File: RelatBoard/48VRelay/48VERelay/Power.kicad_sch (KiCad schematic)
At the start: 25 parts, among them J1 12, U4 3A 32V, U5 TPS630701RNMR, U7 AP7343DQ-33W5-7, U8 AP7343DQ-33W5-7

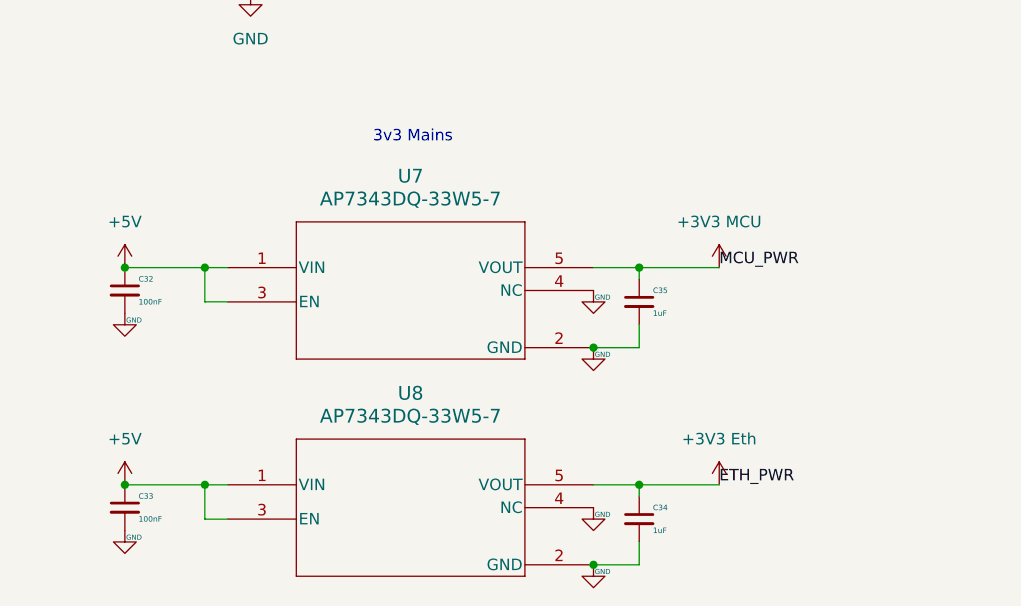
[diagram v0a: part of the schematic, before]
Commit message: begin pcb design
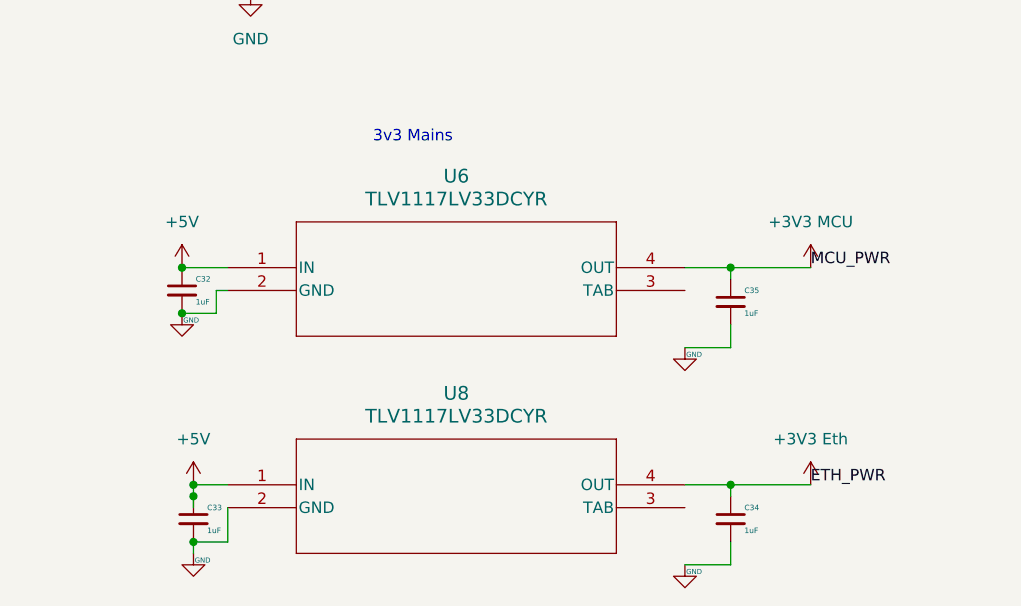
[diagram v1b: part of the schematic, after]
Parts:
- removed U7, U8: AP7343DQ-33W5-7, AP7343DQ-33W5-7_DIO, symbol AP7343DQ-33W5-7:AP7343DQ-33W5-7
- added U6, U8: TLV1117LV33DCYR, YDC4, symbol 2026-06-15_04-40-12:TLV1117LV33DCYR
- C10, C25, C9: footprint (none) -> Capacitor_SMD:C_0201_0603Metric
- C24, C34, C35: footprint (none) -> Capacitor_SMD:C_0805_2012Metric
- C26, C27, C28, C29: footprint CAP_CL21_SAM -> Capacitor_SMD:C_0805_2012Metric
- C30, C31: footprint CAP_CL21_SAM -> Capacitor_SMD:C_1206_3216Metric
- C32, C33: value 100nF -> 1uF; footprint (none) -> Capacitor_SMD:C_0201_0603Metric
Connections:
- net +3V3 Eth: now also U8.4 (OUT)
- net +3V3 MCU: now also U6.4 (OUT)
- net +5V: now also U6.1 (IN), U8.1 (IN)
- net GND: now also U6.2 (GND), U8.2 (GND)
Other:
- moved on the sheet: C32, C33, C34, C35
